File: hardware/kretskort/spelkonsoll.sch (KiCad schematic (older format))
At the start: 2 parts, among them U2 ESP32-DEVKITC-32D, U3 ILI9488

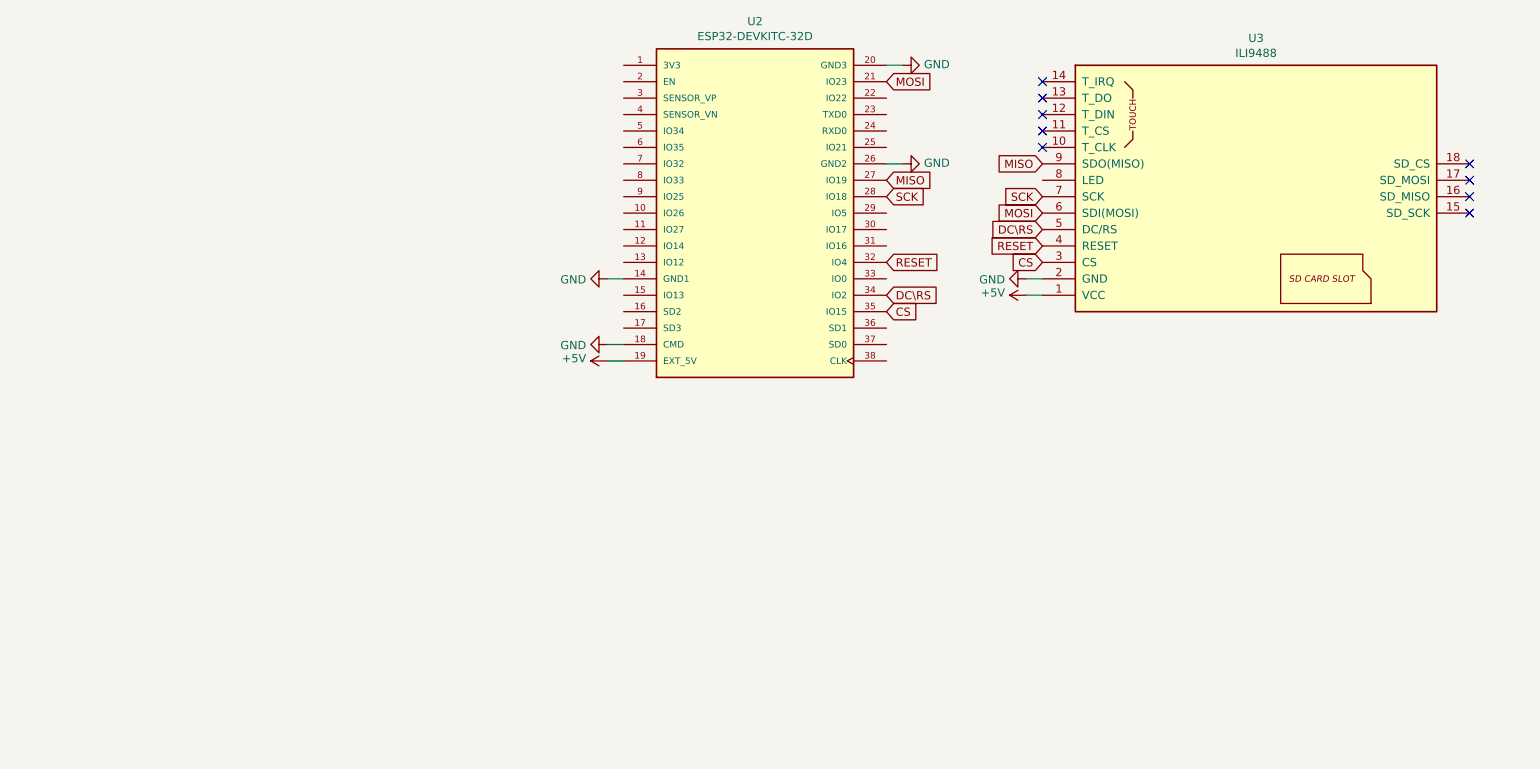
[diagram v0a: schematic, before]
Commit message: more circuit board kicad files
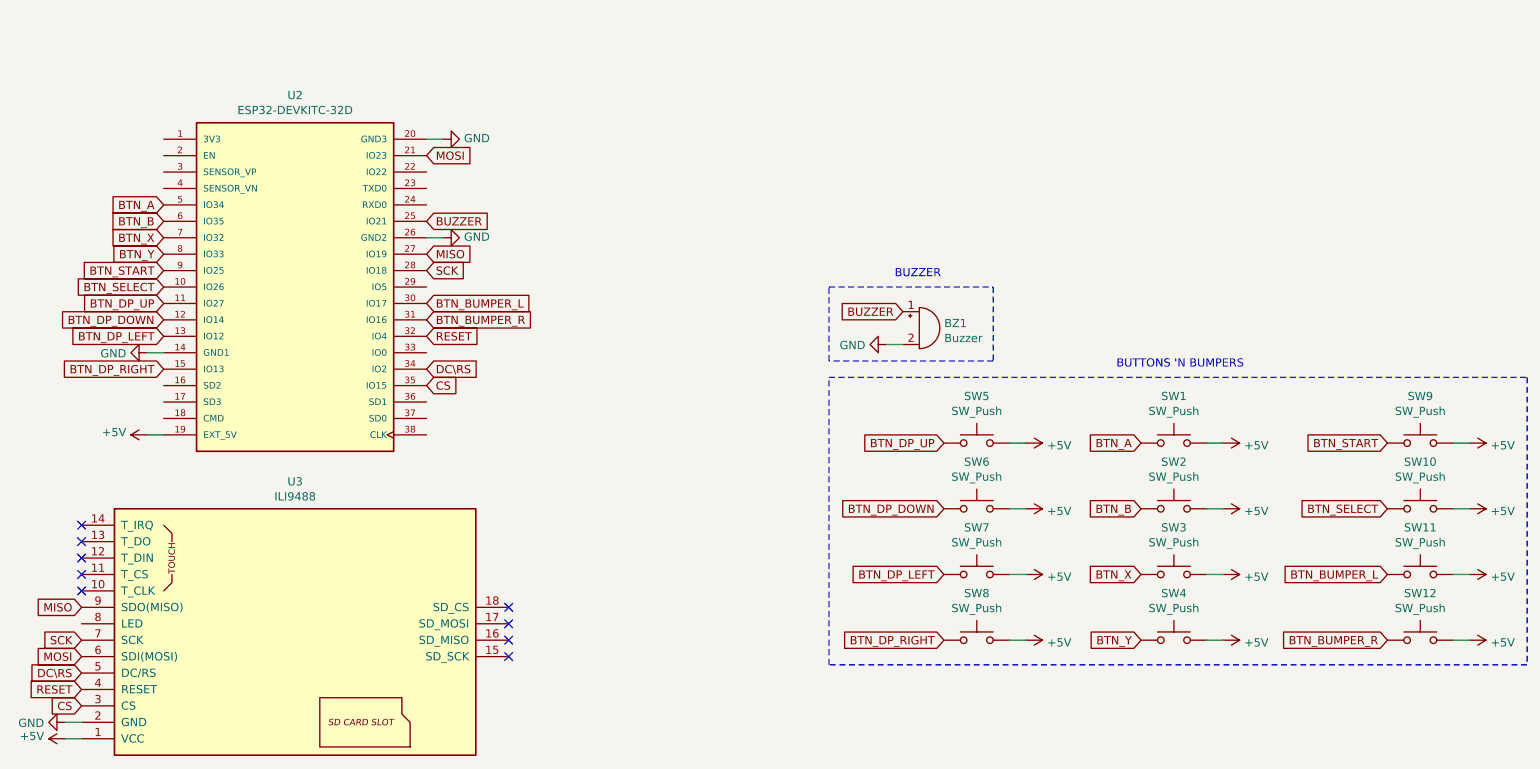
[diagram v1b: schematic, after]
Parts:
- added BZ1: Buzzer, Buzzer_Beeper:Buzzer_15x7.5RM7.6, symbol Device:Buzzer
- added SW1, SW10, SW2, SW3, SW4, SW5, SW6, SW7, SW8, SW9: SW_Push, Button_Switch_THT:SW_TH_Tactile_Omron_B3F-10xx, symbol Switch:SW_Push
- added SW11, SW12: SW_Push, Button_Switch_THT:SW_Tactile_SPST_Angled_PTS645Vx83-2LFS, symbol Switch:SW_Push
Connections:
- net +5V: now also SW1.2, SW10.2, SW11.2, SW12.2, SW2.2, SW3.2, SW4.2, SW5.2, SW6.2, SW7.2, SW8.2, SW9.2
- net GND: now also BZ1.2 (+); no longer U2.18 (CMD)
- net BTN_SELECT: now reaches U2.10 (IO26)
- net BTN_SELECT: now also SW10.1
- net BTN_DP_UP: now reaches U2.11 (IO27)
- net BTN_DP_UP: now also SW5.1
- net BTN_DP_DOWN: now reaches U2.12 (IO14)
- net BTN_DP_DOWN: now also SW6.1
- net BTN_DP_LEFT: now reaches U2.13 (IO12)
- net BTN_DP_LEFT: now also SW7.1
- net BTN_DP_RIGHT: now reaches U2.15 (IO13)
- net BTN_DP_RIGHT: now also SW8.1
- net BUZZER: now reaches U2.25 (IO21)
- net BUZZER: now also BZ1.1 (-)
- net BTN_BUMPER_L: now reaches U2.30 (IO17)
- net BTN_BUMPER_L: now also SW11.1
- net BTN_BUMPER_R: now reaches U2.31 (IO16)
- net BTN_BUMPER_R: now also SW12.1
- net BTN_A: now reaches U2.5 (IO34)
- net BTN_A: now also SW1.1
- net BTN_B: now reaches U2.6 (IO35)
- net BTN_B: now also SW2.1
- net BTN_X: now reaches U2.7 (IO32)
- net BTN_X: now also SW3.1
- net BTN_Y: now reaches U2.8 (IO33)
- net BTN_Y: now also SW4.1
- net BTN_START: now reaches U2.9 (IO25)
- net BTN_START: now also SW9.1
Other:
- note added: "BUTTONS 'N BUMPERS"
- note added: "BUZZER"
- moved on the sheet: U2, U3
